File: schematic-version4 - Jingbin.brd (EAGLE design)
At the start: 47 x 28 mm, 54 parts, among them J2 FTDI_DEVICE, M1 WIRELESS-NRF24L01, Q1 NX3225GD, T1 NMOS, T2 NMOS, T3 NMOS, T4 NMOS, U1 ATMEGA328P_TQFP, U2 GY-521MPU6050

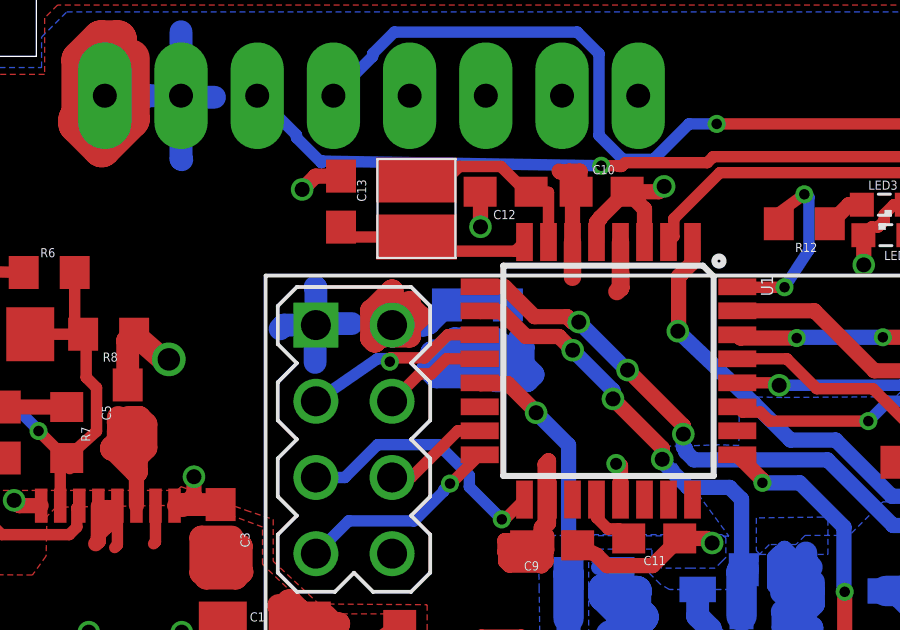
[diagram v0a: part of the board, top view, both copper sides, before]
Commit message: I swear it's the last time
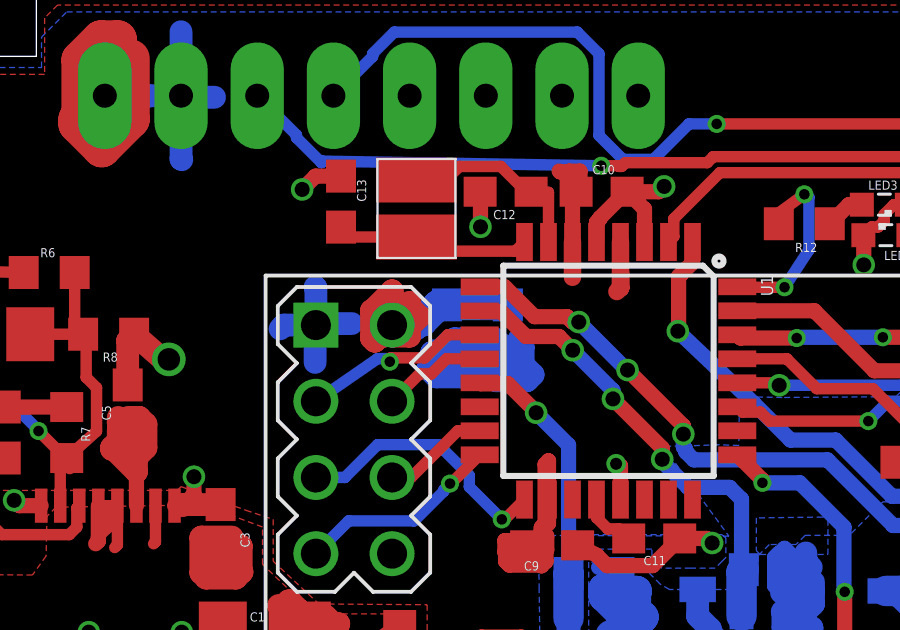
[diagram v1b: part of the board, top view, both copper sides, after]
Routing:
- net V_REG_OUT: track 52.7 -> 53.7 mm
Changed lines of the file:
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@@
 <wire x1="23.9712" y1="19.812" x2="23.9776" y2="19.8056" width="0.508" layer="1"/>
 <wire x1="23.9776" y1="19.8056" x2="23.9776" y2="18.7706" width="0.508" layer="1"/>
-<wire x1="20.2184" y1="17.7156" x2="18.1864" y2="17.7156" width="0.762" layer="16"/>
-<wire x1="18.1864" y1="17.7156" x2="17.5698" y2="17.099" width="0.762" layer="16"/>
-<wire x1="17.5698" y1="17.099" x2="17.46545625" y2="17.099" width="0.762" layer="16"/>
-<wire x1="17.46545625" y1="17.099" x2="17.40985625" y2="17.0434" width="0.762" layer="16"/>
 <wire x1="17.40985625" y1="17.0434" x2="16.3576" y2="17.0434" width="0.762" layer="16"/>
 <wire x1="16.3576" y1="17.0434" x2="16.3576" y2="18.1864" width="0.762" layer="1"/>
@@
 <wire x1="16.9418" y1="17.653" x2="16.9418" y2="17.8054" width="0.762" layer="1"/>
 <wire x1="15.6718" y1="17.526" x2="15.6718" y2="16.6116" width="0.762" layer="1"/>
+<wire x1="20.2184" y1="17.7156" x2="18.1864" y2="17.7156" width="1.016" layer="16"/>
+<wire x1="18.1864" y1="17.7156" x2="17.90245625" y2="17.7156" width="1.016" layer="16"/>
+<wire x1="17.90245625" y1="17.7156" x2="17.35725625" y2="17.1704" width="1.016" layer="16"/>
+<wire x1="17.35725625" y1="17.1704" x2="17.2470375" y2="17.1704" width="1.016" layer="16"/>
+<wire x1="17.2470375" y1="17.1704" x2="17.1200375" y2="17.0434" width="1.016" layer="16"/>
+<wire x1="17.1200375" y1="17.0434" x2="16.3576" y2="17.0434" width="1.016" layer="16"/>
 </signal>
 <signal name="V_BAT">

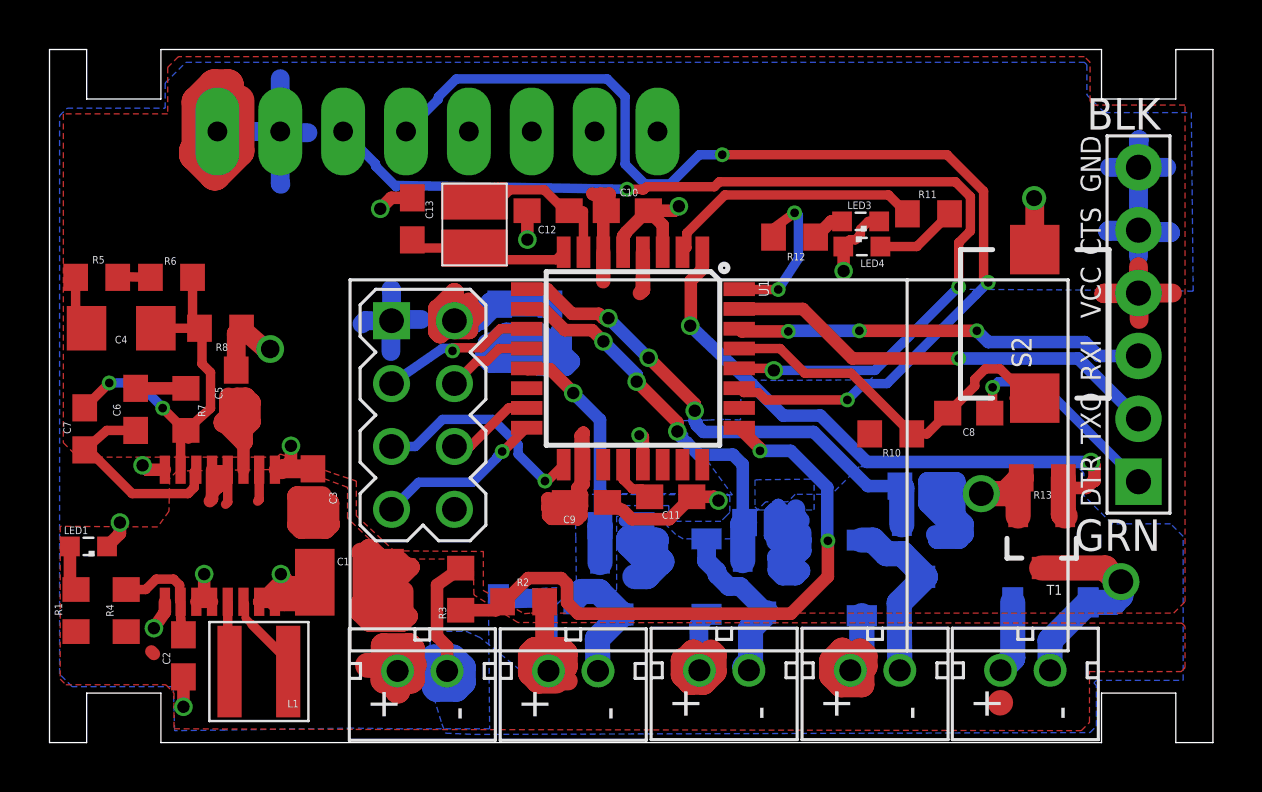
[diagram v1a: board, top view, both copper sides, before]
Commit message: More paths...
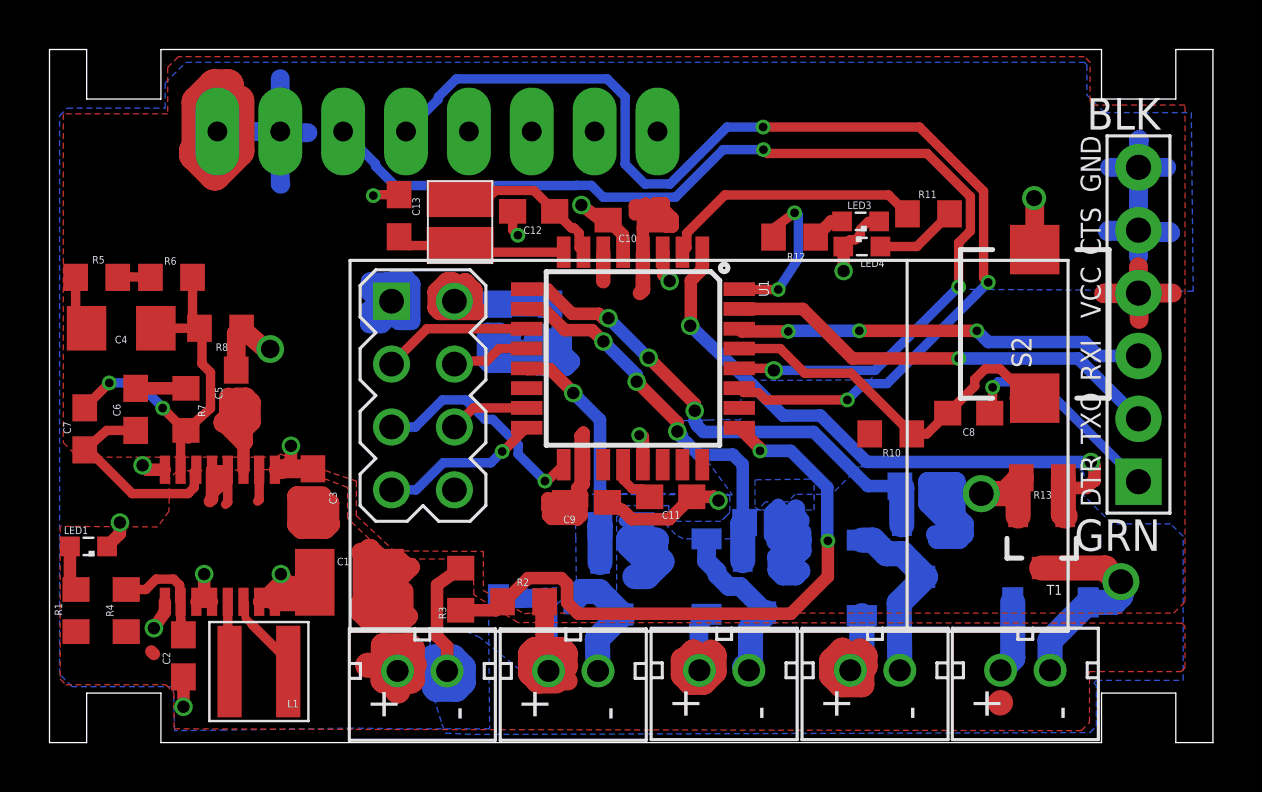
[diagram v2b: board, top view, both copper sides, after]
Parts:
- moved M1 0.79 mm to (26.5, 11.5)
- moved Q1 0.59 mm to (16.6, 21.0)
- moved C12 0.58 mm to (19.6, 21.5)
- moved C13 0.55 mm to (14.1, 21.3)
- moved C10 0.39 mm to (23.4, 21.1), turned to 180 degrees
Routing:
- net GND: track 111.1 -> 113.8 mm, vias 16 -> 17
- net SCL: track 40.9 -> 42.2 mm
- net V_REG_OUT: track 53.7 -> 54.9 mm
- net SDA: track 44.7 -> 45.6 mm
- net CE: track 6.37 -> 6.05 mm, vias 1 -> 0
